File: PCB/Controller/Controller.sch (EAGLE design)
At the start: 109 parts, among them IC2 LMV358IDGKR, Q2 16M

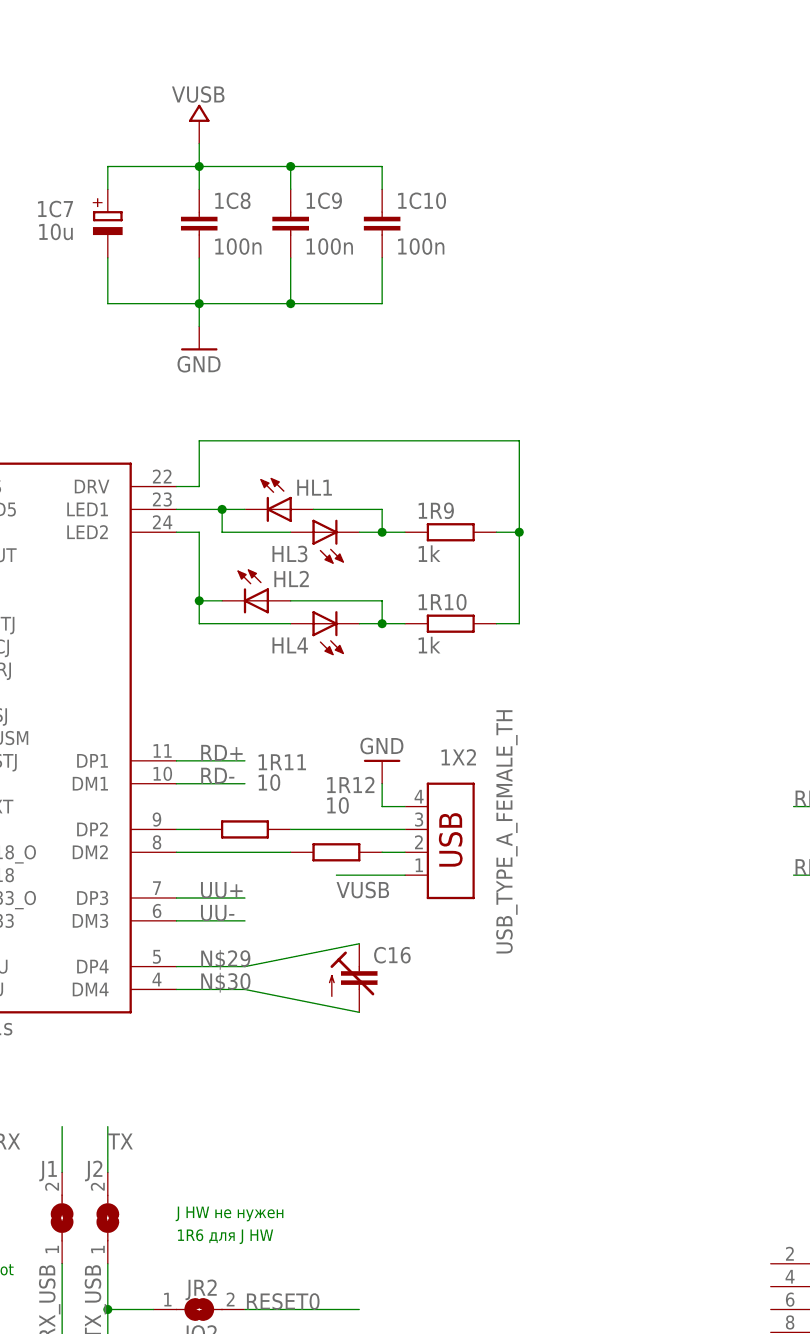
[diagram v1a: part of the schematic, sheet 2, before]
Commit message: pcb c
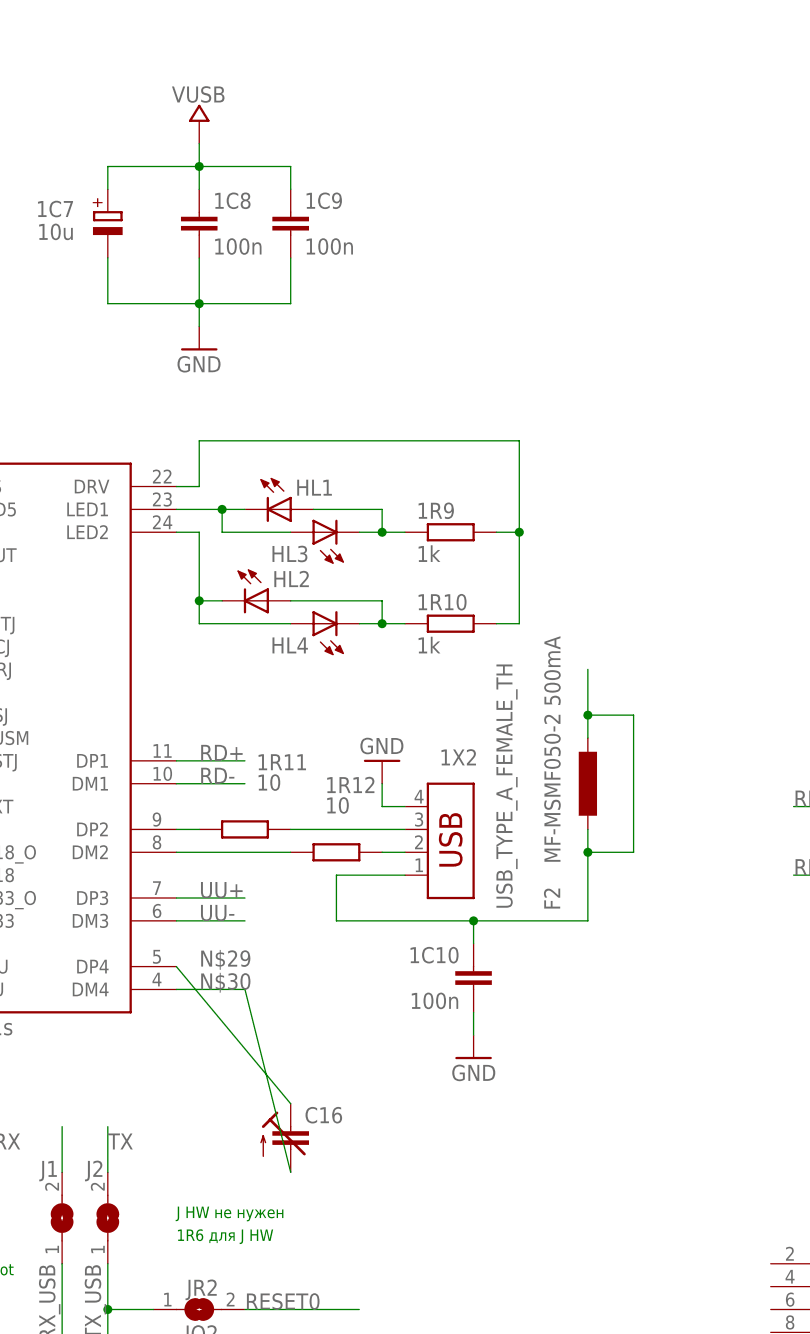
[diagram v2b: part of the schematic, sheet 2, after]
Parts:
- added F2: MF-MSMF050-2 500mA, rcl:L-EUL1812
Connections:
- new net VUSBH: 1C10.1, 1X2.1, F2.1, F2.2
- net GND: now also 1C10.2; no longer 1C10.1
- net VUSB: no longer 1C10.2, 1X2.1
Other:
- moved on the sheet: 1C10, C16
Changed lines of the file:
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@@
 <part name="U_U3" library="jumper" deviceset="SJ" device=""/>
 <part name="U_U4" library="jumper" deviceset="SJ" device=""/>
+<part name="F2" library="rcl" deviceset="L-EU" device="L1812" value="MF-MSMF050-2 500mA"/>
+<part name="GND29" library="supply1" deviceset="GND" device=""/>
 </parts>
 <sheets>
@@
 <instance part="2D3" gate="A" x="548.64" y="246.38"/>
 <instance part="2D3" gate="B" x="543.56" y="215.9"/>
-<instance part="C16" gate="G$1" x="490.22" y="284.48"/>
+<instance part="C16" gate="G$1" x="482.6" y="266.7"/>
 <instance part="1C9" gate="G$1" x="482.6" y="365.76" smashed="yes" rot="MR180">
 <attribute name="NAME" x="484.124" y="370.459" size="1.778" layer="95" rot="MR180"/>
@@
 <instance part="1X2" gate="G$1" x="500.38" y="299.72" smashed="yes" rot="MR180">
 <attribute name="NAME" x="499.11" y="308.61" size="1.778" layer="95" rot="MR180"/>
-<attribute name="VALUE" x="505.46" y="285.75" size="1.778" layer="96" rot="MR90"/>
+<attribute name="VALUE" x="505.46" y="290.83" size="1.778" layer="96" rot="MR90"/>
 </instance>
 <instance part="GND28" gate="1" x="492.76" y="307.34" rot="MR180"/>
@@
 <attribute name="VALUE" x="546.1" y="298.45" size="1.778" layer="96"/>
 </instance>
-<instance part="1C10" gate="G$1" x="492.76" y="365.76" smashed="yes" rot="MR180">
-<attribute name="NAME" x="494.284" y="370.459" size="1.778" layer="95" rot="MR180"/>
-<attribute name="VALUE" x="494.284" y="365.379" size="1.778" layer="96" rot="MR180"/>
-</instance>
+<instance part="1C10" gate="G$1" x="502.92" y="284.48" rot="MR0"/>
 <instance part="1R11" gate="G$1" x="477.52" y="299.72" smashed="yes">
 <attribute name="NAME" x="478.79" y="306.2986" size="1.778" layer="95"/>
@@
 <attribute name="VALUE" x="694.69" y="63.5" size="1.778" layer="96" rot="R90"/>
 </instance>
+<instance part="F2" gate="G$1" x="515.62" y="304.8" smashed="yes">
+<attribute name="NAME" x="510.7686" y="293.37" size="1.778" layer="95" rot="R270"/>
+<attribute name="VALUE" x="512.572" y="295.91" size="1.778" layer="96" rot="R90"/>
+</instance>
+<instance part="GND29" gate="1" x="502.92" y="274.32" rot="MR0"/>
 </instances>
 <busses>
@@
 <wire x1="482.6" y1="363.22" x2="482.6" y2="358.14" width="0.1524" layer="91"/>
 <wire x1="482.6" y1="358.14" x2="472.44" y2="358.14" width="0.1524" layer="91"/>
-<pinref part="1C10" gate="G$1" pin="1"/>
-<wire x1="492.76" y1="363.22" x2="492.76" y2="358.14" width="0.1524" layer="91"/>
-<wire x1="492.76" y1="358.14" x2="482.6" y2="358.14" width="0.1524" layer="91"/>
-<junction x="482.6" y="358.14"/>
 </segment>
 <segment>
@@
 <wire x1="492.76" y1="302.26" x2="492.76" y2="304.8" width="0.1524" layer="91"/>
 </segment>
+<segment>
+<pinref part="1C10" gate="G$1" pin="2"/>
+<pinref part="GND29" gate="1" pin="GND"/>
+<wire x1="502.92" y1="279.4" x2="502.92" y2="276.86" width="0.1524" layer="91"/>
+</segment>
 </net>
 <net name="CD3" class="0">
@@
 <pinref part="1C9" gate="G$1" pin="2"/>
 <wire x1="482.6" y1="373.38" x2="482.6" y2="370.84" width="0.1524" layer="91"/>
-<wire x1="482.6" y1="373.38" x2="492.76" y2="373.38" width="0.1524" layer="91"/>
-<pinref part="1C10" gate="G$1" pin="2"/>
-<wire x1="492.76" y1="373.38" x2="492.76" y2="370.84" width="0.1524" layer="91"/>
-<junction x="482.6" y="373.38"/>
 </segment>
 <segment>
@@
 <wire x1="388.62" y1="309.88" x2="388.62" y2="314.96" width="0.1524" layer="91"/>
 <label x="386.08" y="317.5" size="1.778" layer="95"/>
-</segment>
-<segment>
-<pinref part="1X2" gate="G$1" pin="1"/>
-<wire x1="495.3" y1="294.64" x2="487.68" y2="294.64" width="0.1524" layer="91"/>
-<label x="487.68" y="292.1" size="1.778" layer="95"/>
 </segment>
 </net>
@@
 <segment>
 <pinref part="1D1" gate="G$1" pin="DP4"/>
-<wire x1="469.9" y1="284.48" x2="477.52" y2="284.48" width="0.1524" layer="91"/>
 <label x="472.44" y="284.48" size="1.778" layer="95"/>
 <pinref part="C16" gate="G$1" pin="E"/>
-<wire x1="477.52" y1="284.48" x2="490.22" y2="287.02" width="0.1524" layer="91"/>
+<wire x1="469.9" y1="284.48" x2="482.6" y2="269.24" width="0.1524" layer="91"/>
 </segment>
 </net>
@@
 <label x="472.44" y="281.94" size="1.778" layer="95"/>
 <pinref part="C16" gate="G$1" pin="A"/>
-<wire x1="490.22" y1="279.4" x2="477.52" y2="281.94" width="0.1524" layer="91"/>
+<wire x1="482.6" y1="261.62" x2="477.52" y2="281.94" width="0.1524" layer="91"/>
 </segment>
 </net>
@@
 </segment>
 </net>
+<net name="VUSBH" class="0">
+<segment>
+<pinref part="1X2" gate="G$1" pin="1"/>
+<wire x1="495.3" y1="294.64" x2="487.68" y2="294.64" width="0.1524" layer="91"/>
+<wire x1="487.68" y1="294.64" x2="487.68" y2="289.56" width="0.1524" layer="91"/>
+<wire x1="487.68" y1="289.56" x2="502.92" y2="289.56" width="0.1524" layer="91"/>
+<pinref part="F2" gate="G$1" pin="2"/>
+<wire x1="502.92" y1="289.56" x2="515.62" y2="289.56" width="0.1524" layer="91"/>
+<wire x1="515.62" y1="289.56" x2="515.62" y2="297.18" width="0.1524" layer="91"/>
+<pinref part="1C10" gate="G$1" pin="1"/>
+<wire x1="515.62" y1="297.18" x2="515.62" y2="299.72" width="0.1524" layer="91"/>
+<wire x1="502.92" y1="289.56" x2="502.92" y2="287.02" width="0.1524" layer="91"/>
+<junction x="502.92" y="289.56"/>
+<wire x1="515.62" y1="297.18" x2="520.7" y2="297.18" width="0.1524" layer="91"/>
+<wire x1="520.7" y1="297.18" x2="520.7" y2="312.42" width="0.1524" layer="91"/>
+<pinref part="F2" gate="G$1" pin="1"/>
+<wire x1="515.62" y1="309.88" x2="515.62" y2="312.42" width="0.1524" layer="91"/>
+<wire x1="515.62" y1="312.42" x2="515.62" y2="317.5" width="0.1524" layer="91"/>
+<wire x1="520.7" y1="312.42" x2="515.62" y2="312.42" width="0.1524" layer="91"/>
+<junction x="515.62" y="312.42"/>
+<junction x="515.62" y="297.18"/>
+</segment>
+</net>
